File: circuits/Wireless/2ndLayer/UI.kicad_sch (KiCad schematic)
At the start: 11 parts, among them SW5 SW_DIP_x04, SW6 SW_SPDT

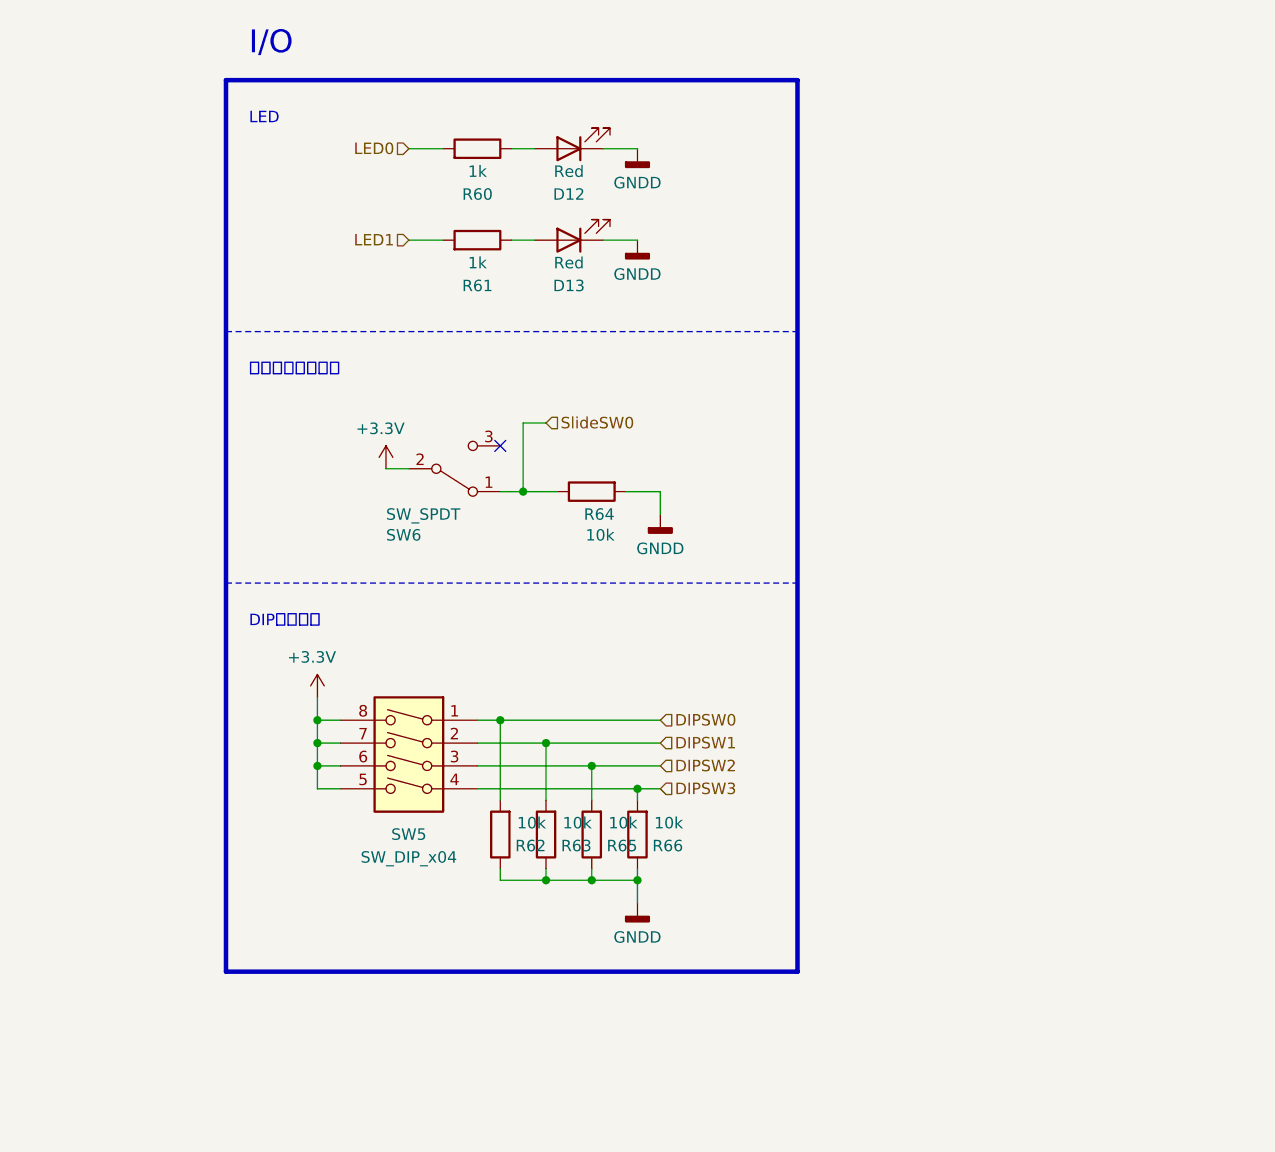
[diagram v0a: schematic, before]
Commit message: PDFプロット
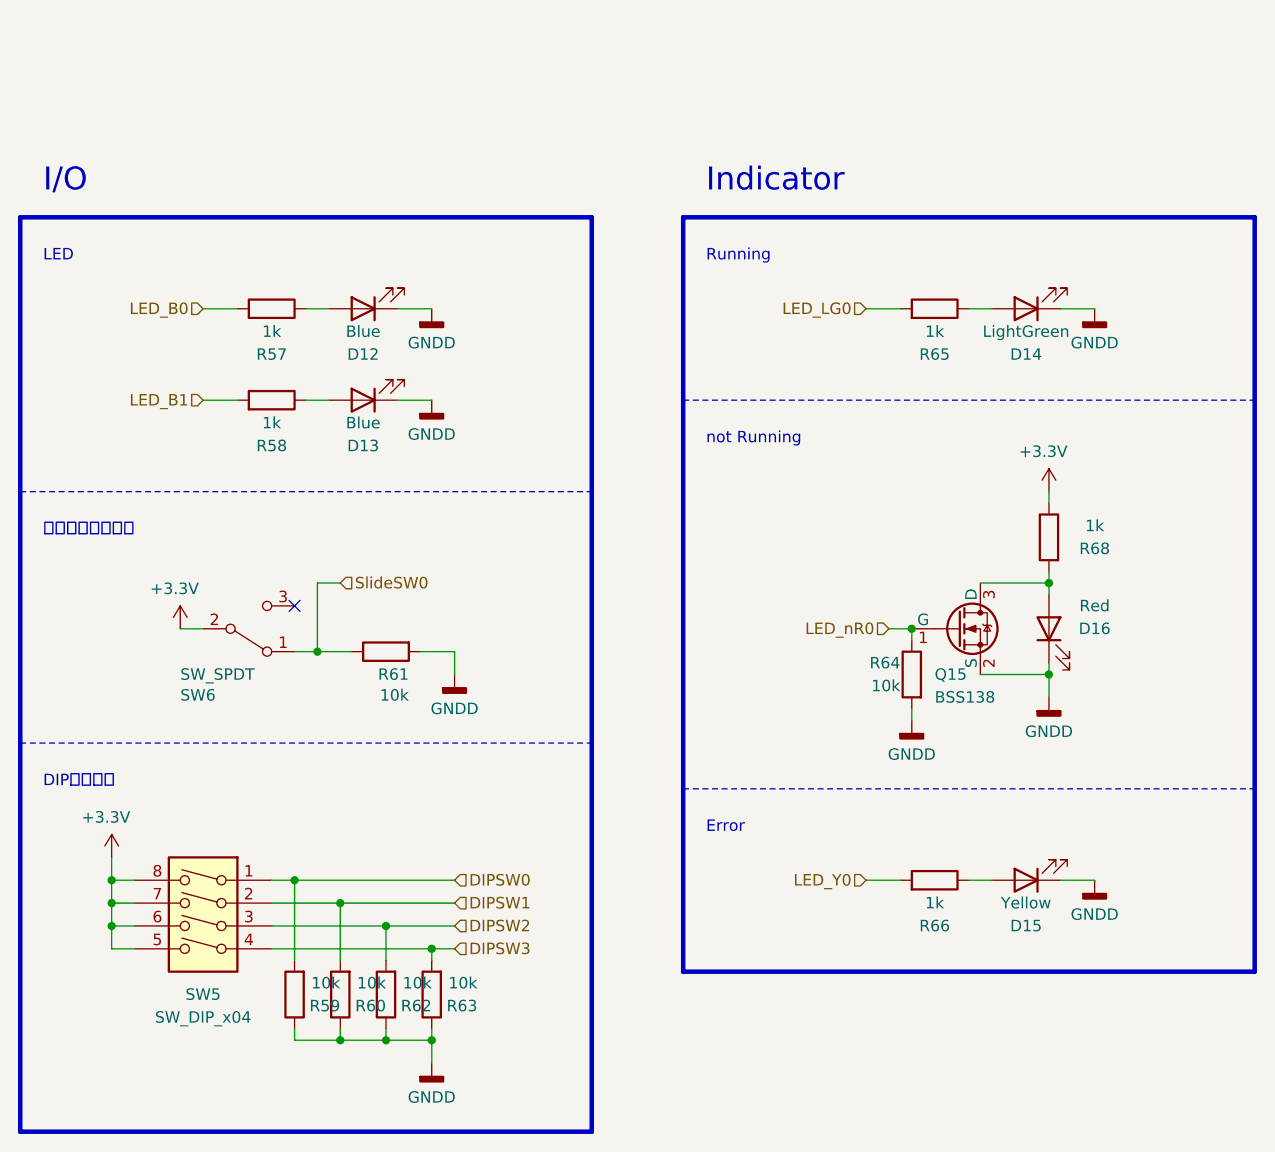
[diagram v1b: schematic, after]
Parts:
- added D14: LightGreen, LED_SMD:LED_0603_1608Metric_Pad1.05x0.95mm_HandSolder, symbol Device:LED
- added D15: Yellow, LED_SMD:LED_0603_1608Metric_Pad1.05x0.95mm_HandSolder, symbol Device:LED
- added D16: Red, LED_SMD:LED_0603_1608Metric_Pad1.05x0.95mm_HandSolder, symbol Device:LED
- added Q15: BSS138, Package_TO_SOT_SMD:SOT-23, symbol Device:Q_NMOS_GSD
- added R57, R58, R68: 1k, Resistor_SMD:R_0402_1005Metric, symbol Device:R
- added R59: 10k, Resistor_SMD:R_0402_1005Metric, symbol Device:R
- D12, D13: value Red -> Blue
- R60, R61: value 1k -> 10k
- R65, R66: value 10k -> 1k
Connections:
- net LED0 is gone; now on net DIPSW1: R60.2
- net LED1 is gone; now on net GNDD: R61.2
- net +3.3V: now also R68.1
- net DIPSW0: now also R59.2; no longer R62.2
- net DIPSW1: no longer R63.2
- net DIPSW2: now also R62.2; no longer R65.2
- net DIPSW3: now also R63.2; no longer R66.2
- net GNDD: now also R60.1, D14.1 (K), D15.1 (K), D16.1 (K), Q15.2 (S), R59.1; no longer R65.1, R66.1
- net SlideSW0: now also R61.1; no longer R64.1
- net at D13.2 (A): now also R58.1; no longer R61.1
- net at D12.2 (A): now also R57.1; no longer R60.1
- new net: D14.2 (A), R65.1
- new net: D15.2 (A), R66.1
- new net: D16.2 (A), Q15.3 (D), R68.2
- new net LED_B0: R57.2
- new net LED_B1: R58.2
- new net LED_LG0: R65.2
- new net LED_Y0: R66.2
- new net LED_nR0: Q15.1 (G), R64.1
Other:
- note added: "Error"
- note added: "Indicator"
- note added: "Running"
- note added: "not Running"

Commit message: シンボル・フットプリントMyLib->TomoshibiLib置き換え
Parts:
- SW6: footprint MyLibrary:SW_Slide_3P_SPDT -> TomoshibiLibrary:SW_Slide_3P_SPDT
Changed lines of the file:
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@@
       (effects (font (size 1.27 1.27)) (justify left))
     )
-    (property "Footprint" "MyLibrary:SW_Slide_3P_SPDT" (at 99.06 101.6 0)
+    (property "Footprint" "TomoshibiLibrary:SW_Slide_3P_SPDT" (at 99.06 101.6 0)
       (effects (font (size 1.27 1.27)) hide)
     )
